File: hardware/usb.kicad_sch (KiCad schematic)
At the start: 35 parts, among them J1 USB_A_Stacked, J2 USB_C_Receptacle_USB2.0_14P, J3 USB_C_Receptacle_USB2.0_14P, J4 USB_C_Receptacle_USB2.0_14P, U10 SY6280AAC, U11 SY6280AAC, U12 SY6280AAC, U13 TPD2EUSB30, U14 TPD2EUSB30, U15 TPD2EUSB30, U16 TPD2EUSB30, U17 HUSB237, U18 TPD2EUSB30, U9 SY6280AAC

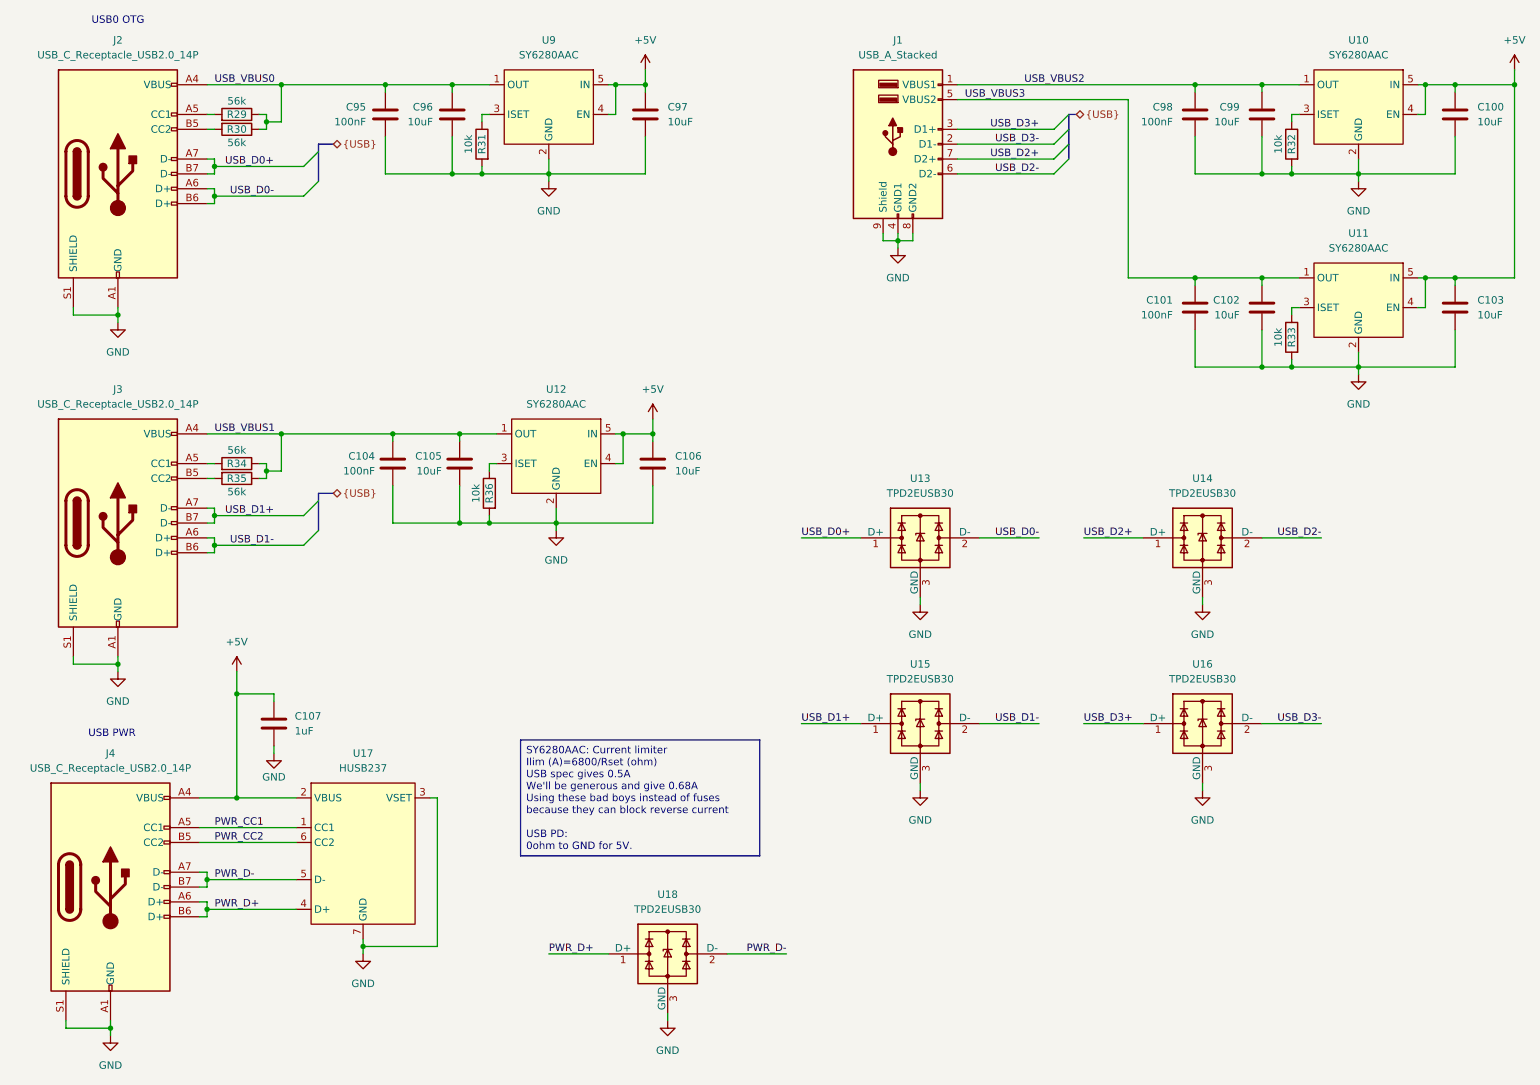
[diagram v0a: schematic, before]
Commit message: Add fixes and improvements
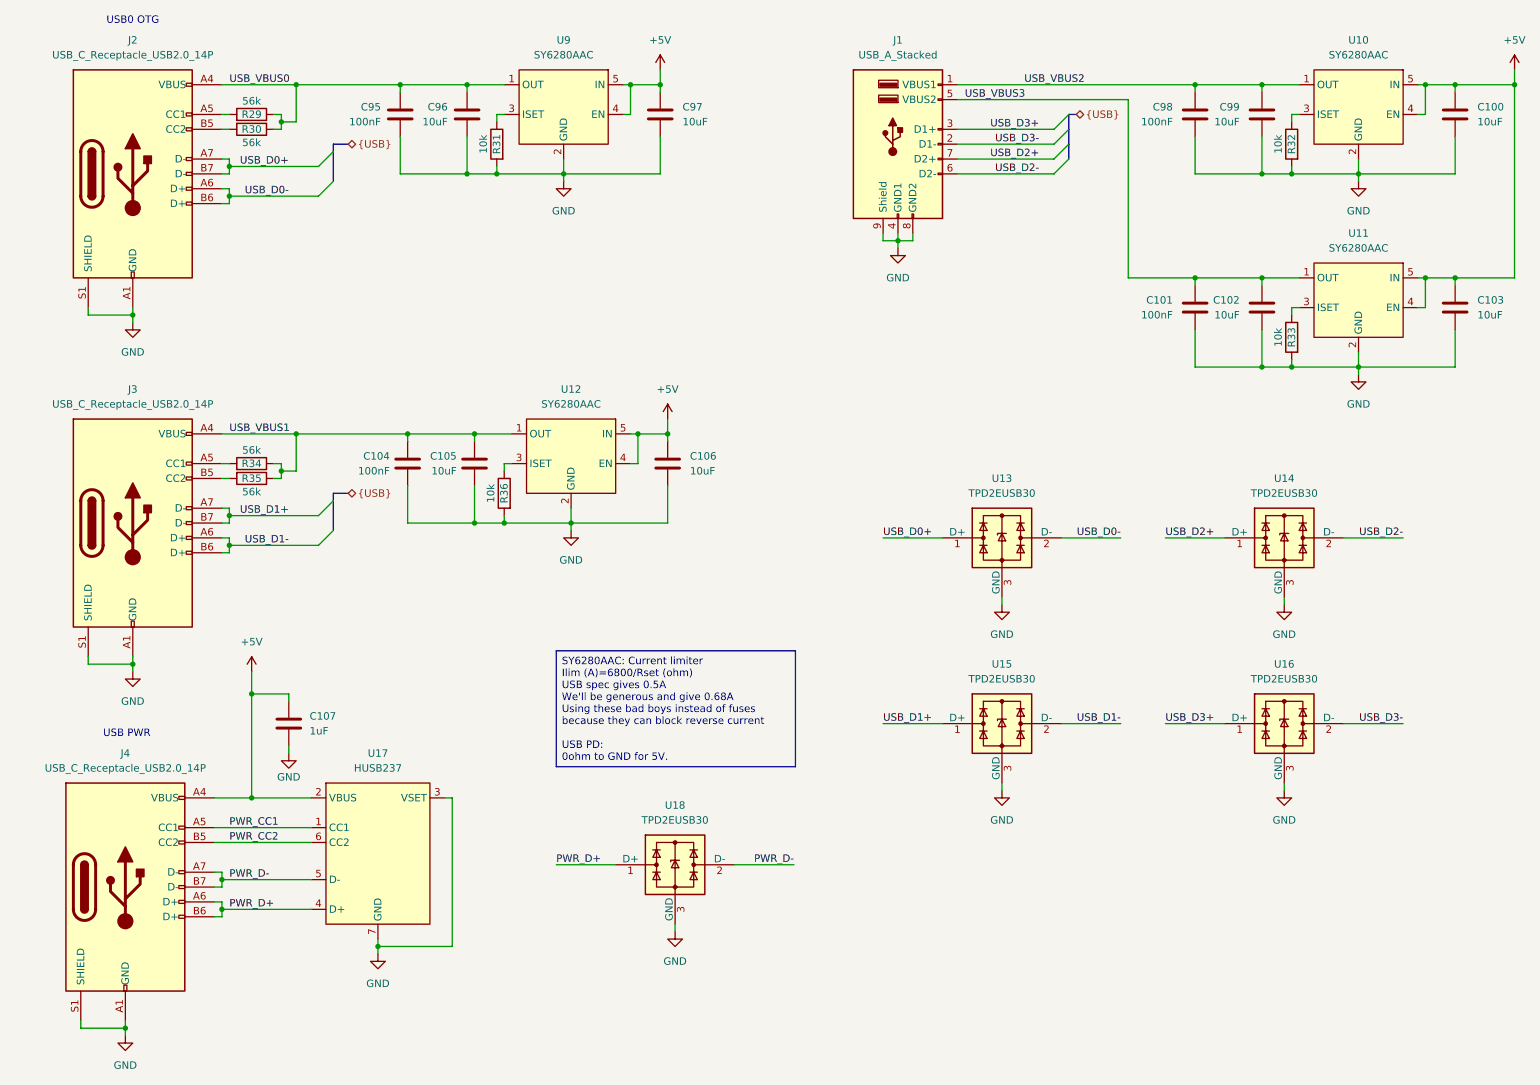
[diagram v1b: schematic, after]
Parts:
- J2, J3, J4: FT Position Offset 0,-12.7 -> 0,12.7
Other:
- moved on the sheet: C104, C105, C106, C107, C95, C96, C97, J2, J3, J4, R29, R30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
